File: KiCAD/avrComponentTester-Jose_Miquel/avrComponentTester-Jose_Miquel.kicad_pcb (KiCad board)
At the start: 2 copper layers, 6 parts, among them J4 3-pin_test_header, U1 ST7735_1.8

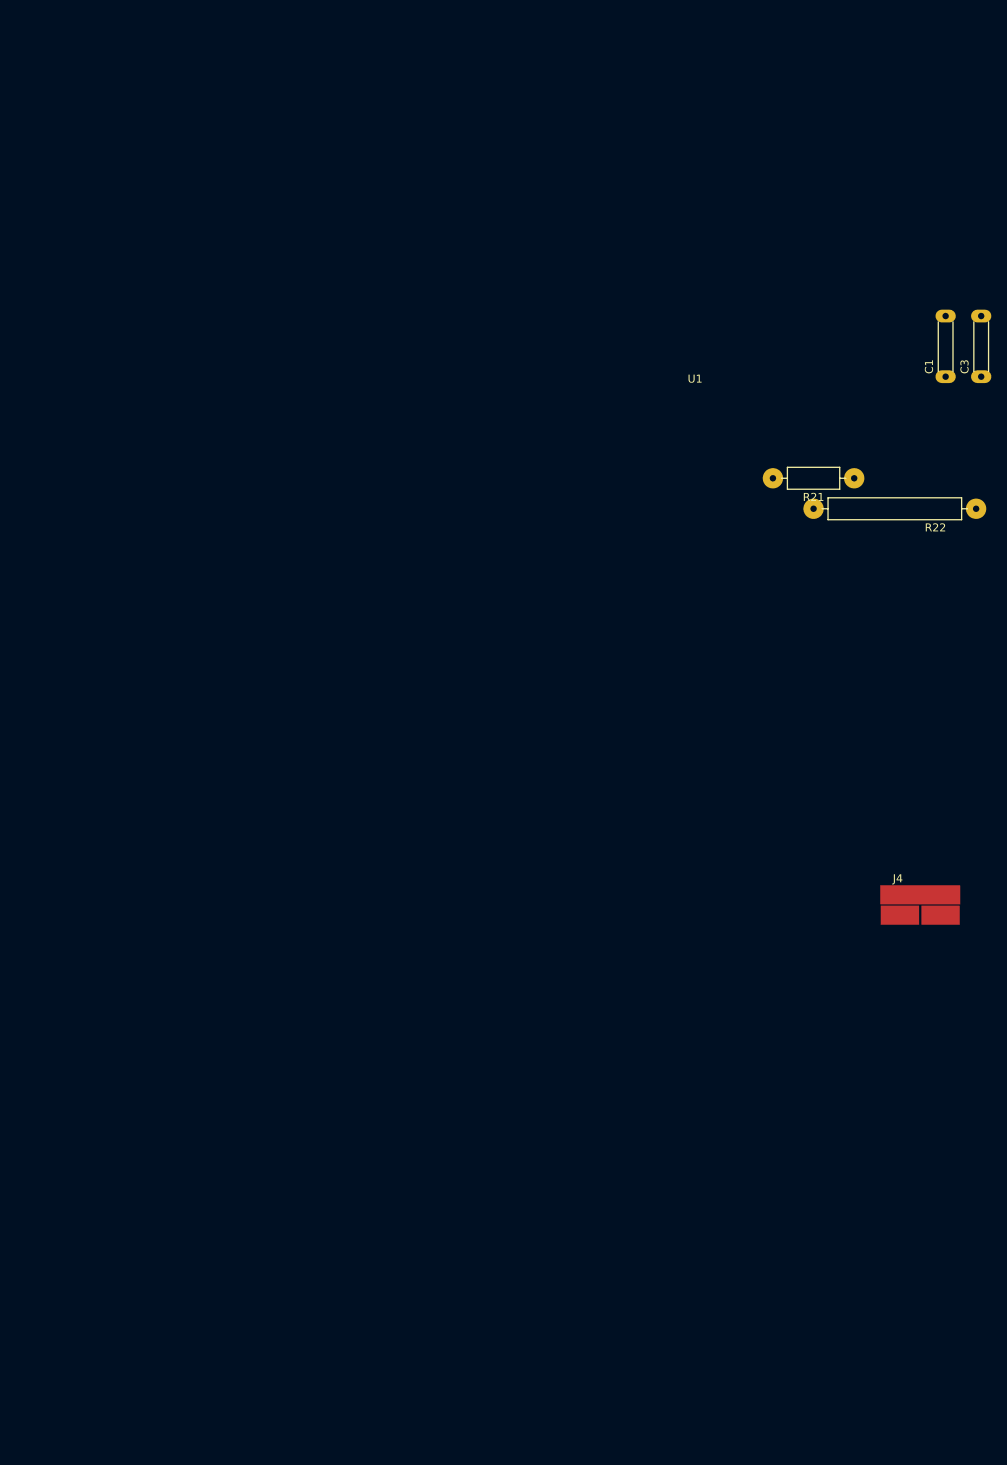
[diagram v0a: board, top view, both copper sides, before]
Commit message: New PCB and some READMEs
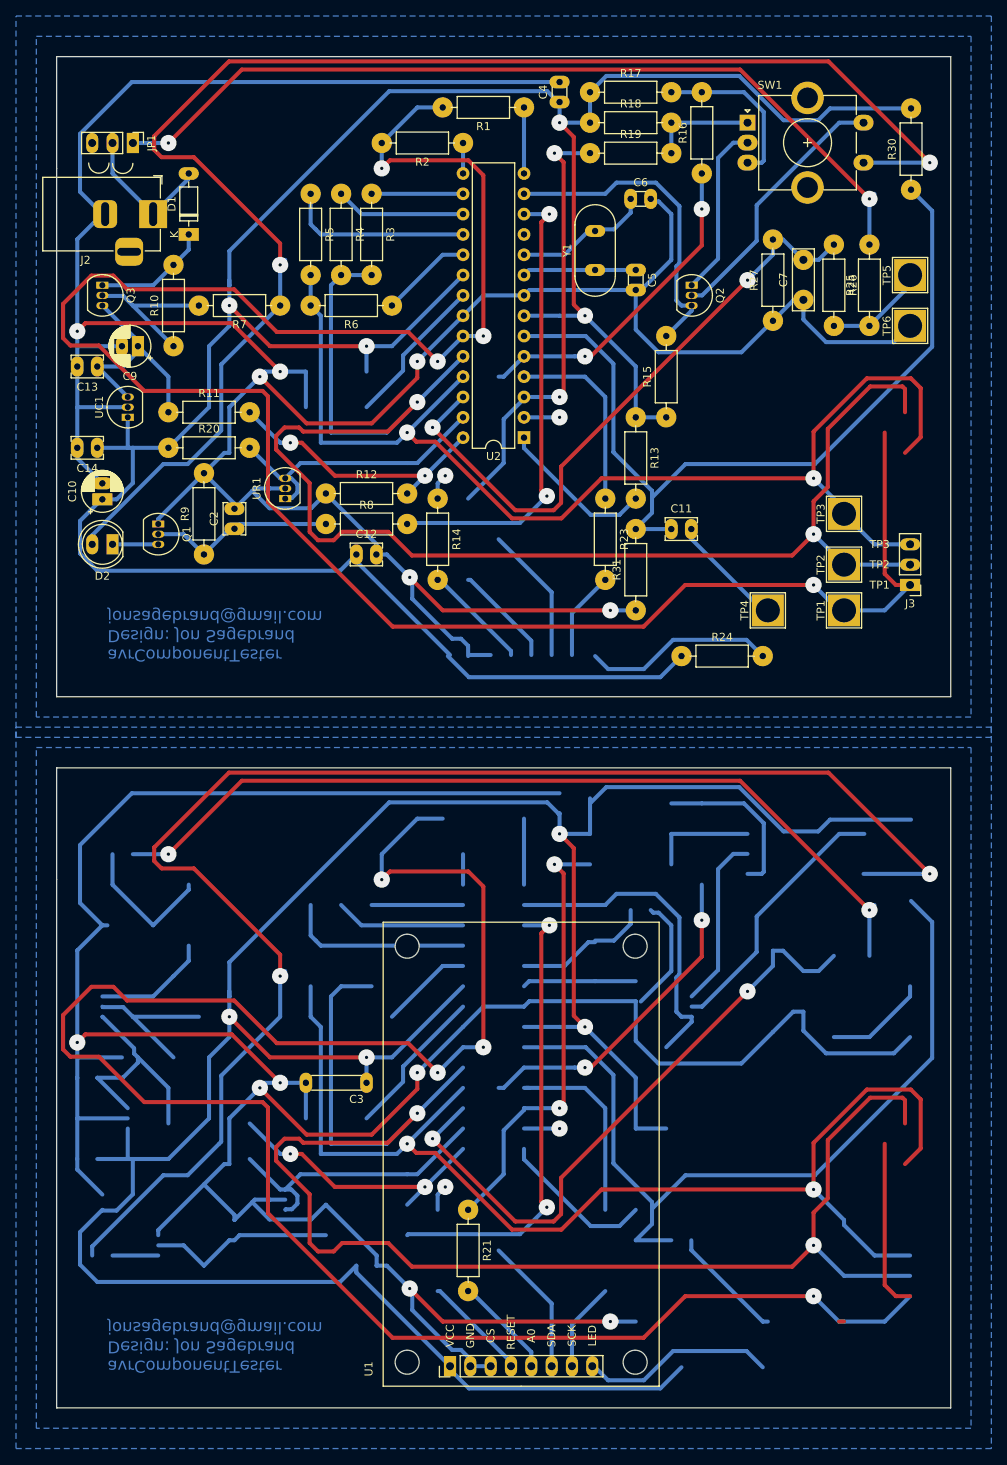
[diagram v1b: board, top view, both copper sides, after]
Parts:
- removed C1: 1n, My_Misc:C_Disc_D3.0mm_W1.6mm_P7.68mm_large
- removed J4: 3-pin_test_header, My_Parts:3-pad_SMD_test-pad
- removed R22: 10k, My_Misc:R_Axial_DIN0207_L6.3mm_D2.5mm_P20.32mm_Horizontal_larger_pads
- added C10: 10u, My_Misc:CP_Radial_D5.0mm_P2.00mm_larger, F.Cu at (28.6, 74.4)
- added C11: 100n, My_Misc:C_Disc_D3.8mm_W2.6mm_P2.50mm_large, F.Cu at (99.7, 78.1)
- added C12: 100n, My_Misc:C_Disc_D3.8mm_W2.6mm_P2.50mm_large, F.Cu at (60.3, 81.3)
- added C13: 100n, My_Misc:C_Disc_D3.8mm_W2.6mm_P2.50mm_large, F.Cu at (27.9, 57.8)
- added C14: 100n, My_Misc:C_Disc_D3.8mm_W2.6mm_P2.50mm_large, F.Cu at (27.9, 67.9)
- added C2: 10n, My_Misc:C_Disc_D3.8mm_W2.6mm_P2.50mm_large, F.Cu at (45.1, 78.1)
- added C4: 100n, My_Misc:C_Disc_D3.0mm_W1.6mm_P2.50mm_larg, F.Cu at (85.7, 24.7)
- added C5: 22p, My_Misc:C_Disc_D3.0mm_W1.6mm_P2.50mm_larg, F.Cu at (95.2, 45.7)
- added C6: 22p, My_Misc:C_Disc_D3.0mm_W1.6mm_P2.50mm_larg, F.Cu at (94.6, 36.8)
- added C7: 10n 100V, My_Misc:C_Disc_D7.5mm_W2.5mm_P5.00mm_larger, F.Cu at (116.2, 49.5)
- added C9: 10u, My_Misc:CP_Radial_D5.0mm_P2.00mm_larger, F.Cu at (33.0, 55.2)
- added D1: D_Schottky, My_Misc:D_DO-35_SOD27_P7.62mm_Horizontal_large, F.Cu at (39.4, 41.3)
- added D2: LED, My_Misc:LED_D5.0mm_larger_pads, F.Cu at (29.8, 80.0)
- added J2: 8-15VDC In, Connector_BarrelJack:BarrelJack_Horizontal, F.Cu at (34.9, 38.7)
- added J3: 3-pin_test_header, My_Headers:3-pin_test_header_large, F.Cu at (129.5, 85.1)
- added JP1: Vext <50V, Zener < VCC, My_Parts:Jumper_1x03_P2.54mm_large, F.Cu at (32.4, 29.8)
- added Q1: 2N3904, My_Misc:TO-92_Inline_large, F.Cu at (35.6, 77.5)
- added Q2: 2N3904, My_Misc:TO-92_Inline_large, F.Cu at (102.2, 47.6)
- added Q3: 2N3906, My_Misc:TO-92_Inline_large, F.Cu at (28.6, 47.6)
- added R1: 680R, My_Misc:R_Axial_DIN0207_L6.3mm_D2.5mm_P10.16mm_Horizontal_larger_pads, F.Cu at (81.3, 25.4)
- added R10: 33k, My_Misc:R_Axial_DIN0207_L6.3mm_D2.5mm_P10.16mm_Horizontal_larger_pads, F.Cu at (37.5, 55.2)
- added R11: 10k, My_Misc:R_Axial_DIN0207_L6.3mm_D2.5mm_P10.16mm_Horizontal_larger_pads, F.Cu at (36.8, 63.5)
- added R12: 3k3, My_Misc:R_Axial_DIN0207_L6.3mm_D2.5mm_P10.16mm_Horizontal_larger_pads, F.Cu at (56.5, 73.7)
- added R13: 10k, My_Misc:R_Axial_DIN0207_L6.3mm_D2.5mm_P10.16mm_Horizontal_larger_pads, F.Cu at (95.2, 64.1)
- added R14: 10k, My_Misc:R_Axial_DIN0207_L6.3mm_D2.5mm_P10.16mm_Horizontal_larger_pads, F.Cu at (70.5, 74.3)
- added R15: 27k, My_Misc:R_Axial_DIN0207_L6.3mm_D2.5mm_P10.16mm_Horizontal_larger_pads, F.Cu at (99.1, 64.1)
- added R16: 1k, My_Misc:R_Axial_DIN0207_L6.3mm_D2.5mm_P10.16mm_Horizontal_larger_pads, F.Cu at (103.5, 33.7)
- added R17: 10k, My_Misc:R_Axial_DIN0207_L6.3mm_D2.5mm_P10.16mm_Horizontal_larger_pads, F.Cu at (89.5, 23.5)
- added R18: 10k, My_Misc:R_Axial_DIN0207_L6.3mm_D2.5mm_P10.16mm_Horizontal_larger_pads, F.Cu at (89.5, 27.3)
- added R19: 1k, My_Misc:R_Axial_DIN0207_L6.3mm_D2.5mm_P10.16mm_Horizontal_larger_pads, F.Cu at (89.5, 31.1)
- added R2: 470k, My_Misc:R_Axial_DIN0207_L6.3mm_D2.5mm_P10.16mm_Horizontal_larger_pads, F.Cu at (73.7, 29.8)
- added R20: 2k2, My_Misc:R_Axial_DIN0207_L6.3mm_D2.5mm_P10.16mm_Horizontal_larger_pads, F.Cu at (36.8, 67.9)
- added R23: 10k, My_Misc:R_Axial_DIN0207_L6.3mm_D2.5mm_P10.16mm_Horizontal_larger_pads, F.Cu at (91.4, 74.3)
- added R24: 220R, My_Misc:R_Axial_DIN0207_L6.3mm_D2.5mm_P10.16mm_Horizontal_larger_pads, F.Cu at (101.0, 94.0)
- added R25: 2k2, My_Misc:R_Axial_DIN0207_L6.3mm_D2.5mm_P10.16mm_Horizontal_larger_pads, F.Cu at (124.5, 52.7)
- added R26: 179k45, My_Misc:R_Axial_DIN0207_L6.3mm_D2.5mm_P10.16mm_Horizontal_larger_pads, F.Cu at (120.0, 42.5)
- added R27: 20k, My_Misc:R_Axial_DIN0207_L6.3mm_D2.5mm_P10.16mm_Horizontal_larger_pads, F.Cu at (112.4, 52.1)
- added R3: 680R, My_Misc:R_Axial_DIN0207_L6.3mm_D2.5mm_P10.16mm_Horizontal_larger_pads, F.Cu at (62.2, 36.2)
- added R30: 10k, My_Misc:R_Axial_DIN0207_L6.3mm_D2.5mm_P10.16mm_Horizontal_larger_pads, F.Cu at (129.7, 35.7)
- added R31: 10k, My_Misc:R_Axial_DIN0207_L6.3mm_D2.5mm_P10.16mm_Horizontal_larger_pads, F.Cu at (95.2, 88.3)
- added R4: 470k, My_Misc:R_Axial_DIN0207_L6.3mm_D2.5mm_P10.16mm_Horizontal_larger_pads, F.Cu at (58.4, 36.2)
- added R5: 680R, My_Misc:R_Axial_DIN0207_L6.3mm_D2.5mm_P10.16mm_Horizontal_larger_pads, F.Cu at (54.6, 36.2)
- added R6: 470k, My_Misc:R_Axial_DIN0207_L6.3mm_D2.5mm_P10.16mm_Horizontal_larger_pads, F.Cu at (64.8, 50.2)
- added R7: 3k3, My_Misc:R_Axial_DIN0207_L6.3mm_D2.5mm_P10.16mm_Horizontal_larger_pads, F.Cu at (50.8, 50.2)
- added R8: 27k, My_Misc:R_Axial_DIN0207_L6.3mm_D2.5mm_P10.16mm_Horizontal_larger_pads, F.Cu at (56.5, 77.5)
- added R9: 100k, My_Misc:R_Axial_DIN0207_L6.3mm_D2.5mm_P10.16mm_Horizontal_larger_pads, F.Cu at (41.3, 81.3)
- added SW1: EC11, My_Misc:RotaryEncoder_Alps_EC11E-Switch_Vertical_H20mm_CircularMountingHoles_large, F.Cu at (109.2, 27.3)
- added TP1: TestPoint, My_Parts:TestPoint_THTPad_4.0x4.0mm_Drill3.0mm, F.Cu at (121.3, 88.3)
- added TP2: TestPoint, My_Parts:TestPoint_THTPad_4.0x4.0mm_Drill3.0mm, F.Cu at (121.3, 82.5)
- added TP3: TestPoint, My_Parts:TestPoint_THTPad_4.0x4.0mm_Drill3.0mm, F.Cu at (121.3, 76.2)
- added TP4: TestPoint, My_Parts:TestPoint_THTPad_4.0x4.0mm_Drill3.0mm, F.Cu at (111.8, 88.3)
- added TP5: TestPoint, My_Parts:TestPoint_THTPad_4.0x4.0mm_Drill3.0mm, F.Cu at (129.5, 46.4)
- added TP6: TestPoint, My_Parts:TestPoint_THTPad_4.0x4.0mm_Drill3.0mm, F.Cu at (129.5, 52.7)
- added U2: ATmega328P-PU, Package_DIP:DIP-28_W7.62mm, F.Cu at (81.3, 66.7)
- added UC1: L78L05_TO92, My_Misc:TO-92_Inline_large, F.Cu at (31.8, 64.1)
- added UR1: TL431LP, My_Misc:TO-92_Inline_large, F.Cu at (51.4, 74.3)
- added Y1: 8MHz, My_Misc:Crystal_HC49-4H_Vertical_large, F.Cu at (90.2, 45.7)
- moved U1 117.4 mm to (72.0, 182.7), turned to 90 degrees
- moved C3 117.0 mm to (61.6, 147.3), turned to 180 degrees
- moved R21 103.4 mm to (74.3, 163.2), turned to 270 degrees
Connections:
- C3 pad 1: +5V -> (no net)
- C3 pad 2: TPGND -> (no net)
- R21 pad 1: A0 -> (no net)
- R21 pad 2: Net-(R21-Pad2) -> (no net)
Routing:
- net (no net): track 0.00 -> 2560.0 mm, vias 0 -> 34
- net TPGND: track 0.00 -> 412.7 mm, vias 0 -> 6
- net +5V: track 0.00 -> 338.5 mm, vias 0 -> 4
- net TP1: track 0.00 -> 266.0 mm, vias 0 -> 4
- net Net-(D2-Pad2): track 0.00 -> 187.4 mm, vias 0 -> 2
- net TP2: track 0.00 -> 186.7 mm, vias 0 -> 2
- net TP3: track 0.00 -> 147.3 mm, vias 0 -> 2
- net Net-(JP1-Pad1): track 0.00 -> 109.8 mm, vias 0 -> 2
- net FreqMeas: track 0.00 -> 104.1 mm
- net ZenerMeas: track 0.00 -> 80.1 mm, vias 0 -> 2
- net Net-(R8-Pad2): track 0.00 -> 58.5 mm, vias 0 -> 2
- net A0: track 0.00 -> 55.6 mm, vias 0 -> 2
- net SDA: track 0.00 -> 41.2 mm, vias 0 -> 2
- net Net-(Q2-Pad3): track 0.00 -> 40.5 mm
- net Net-(R20-Pad2): track 0.00 -> 36.1 mm
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- added copper zone on B.Cu, net (none)
- added copper zone on B.Cu, net TPGND
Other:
- board outline added: 111.8 x 168.9 mm
- board text added: "avrComponentTester Design: Jon Sagebrand jonsagebrand@gmail.com"
